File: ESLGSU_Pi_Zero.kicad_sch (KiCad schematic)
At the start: 1 part

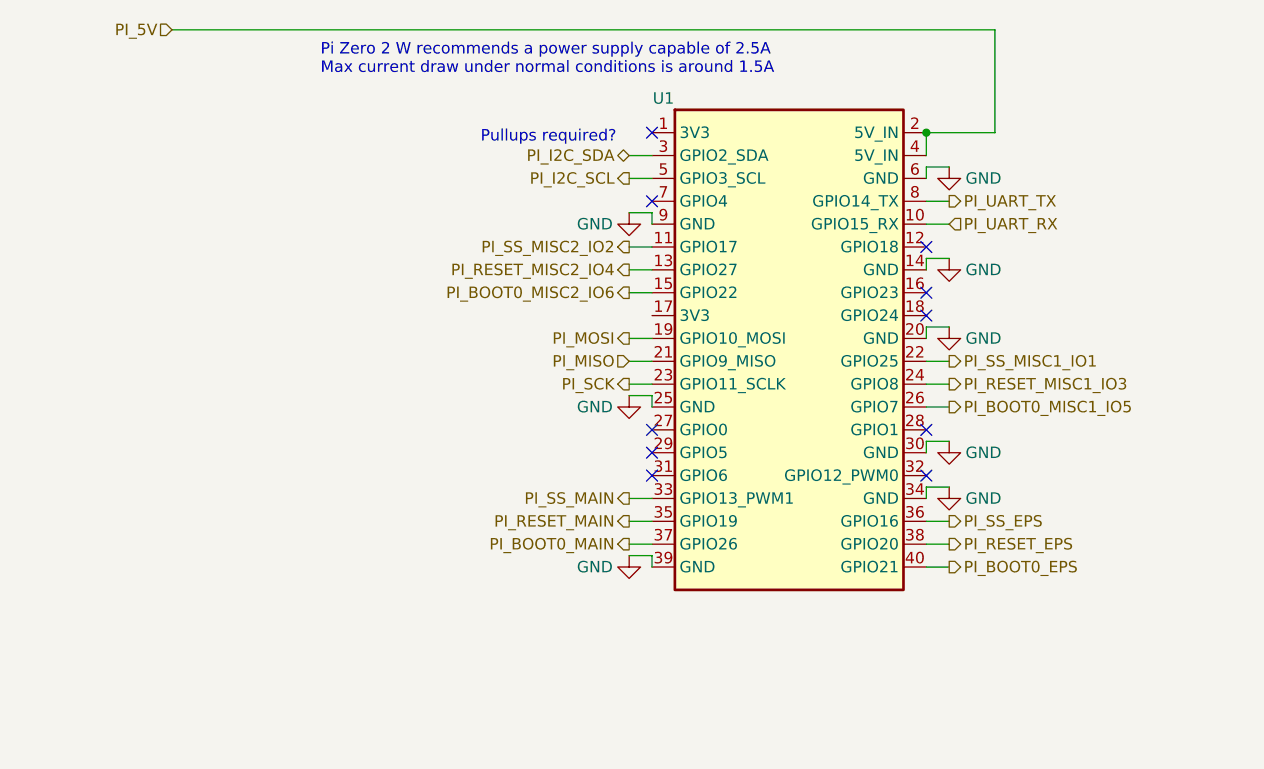
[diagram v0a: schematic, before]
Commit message: Started work on system power section
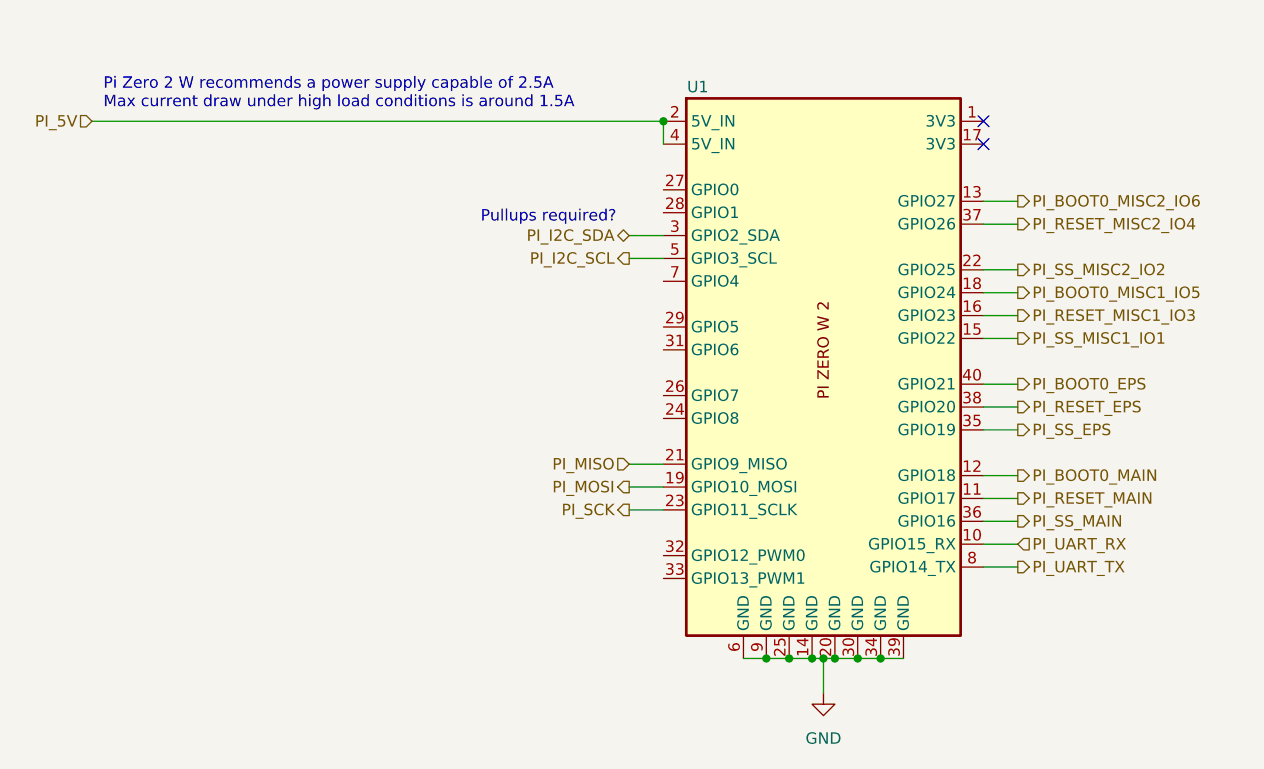
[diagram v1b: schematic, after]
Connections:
- net PI_BOOT0_MAIN: now also U1.12 (GPIO18); no longer U1.37 (GPIO26)
- net PI_BOOT0_MISC1_IO5: now also U1.18 (GPIO24); no longer U1.26 (GPIO7)
- net PI_BOOT0_MISC2_IO6: now also U1.13 (GPIO27); no longer U1.15 (GPIO22)
- net PI_RESET_MAIN: now also U1.11 (GPIO17); no longer U1.35 (GPIO19)
- net PI_RESET_MISC1_IO3: now also U1.16 (GPIO23); no longer U1.24 (GPIO8)
- net PI_RESET_MISC2_IO4: now also U1.37 (GPIO26); no longer U1.13 (GPIO27)
- net PI_SS_EPS: now also U1.35 (GPIO19); no longer U1.36 (GPIO16)
- net PI_SS_MAIN: now also U1.36 (GPIO16); no longer U1.33 (GPIO13_PWM1)
- net PI_SS_MISC1_IO1: now also U1.15 (GPIO22); no longer U1.22 (GPIO25)
- net PI_SS_MISC2_IO2: now also U1.22 (GPIO25); no longer U1.11 (GPIO17)
- no-connect marks 10 -> 2
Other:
- note added: "Pi Zero 2 W recommends a power supply capable of 2.5A Max current draw under high load conditions is around 1.5A"
- note removed: "Pi Zero 2 W recommends a power supply capable of 2.5A Max current draw under normal conditions is around 1.5A"
